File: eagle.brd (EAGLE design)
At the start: 65 x 56 mm, 11 parts, among them IC1 74HCT245, IC2 74HCT245

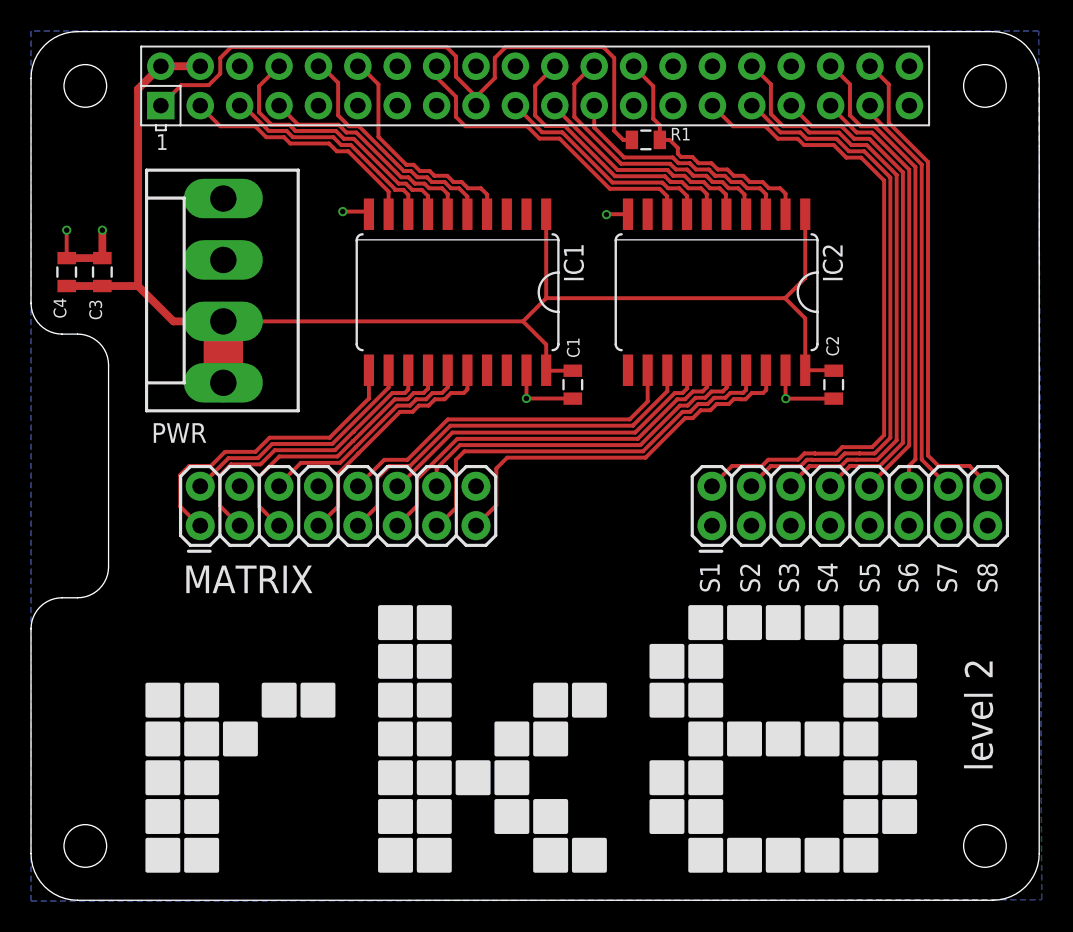
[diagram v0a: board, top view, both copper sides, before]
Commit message: level 3 design
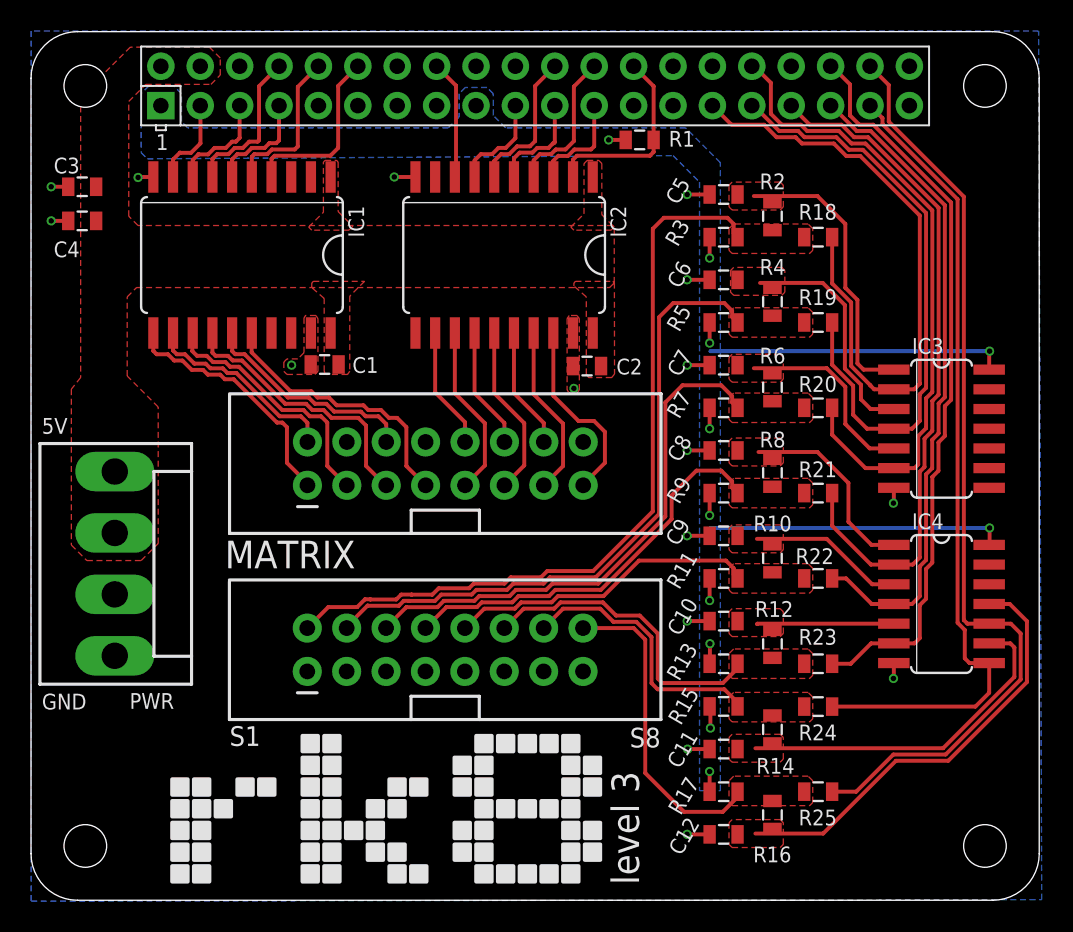
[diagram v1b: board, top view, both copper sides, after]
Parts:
- added C10, C11, C12, C5, C6, C7, C8, C9: 0.1uF, passive:0805
- added IC3, IC4: 74HC14D, 74xx-eu:SO14
- added R10, R11, R12, R13, R14, R15, R16, R17, R2, R3, R4, R5, R6, R7, R8, R9: 10K, passive:0805
- added R18, R19, R20, R21, R22, R23, R24, R25: 0, passive:0805
- J1, J2: device SparkFun-Connectors:2X8 -> SparkFun-Connectors:2X8-SHROUDED_LOCK
- U$1: value RPI3_HATNO_CF -> RPI3_HATNO_DF; device rpi:RASPI_BOARD_B+HAT_DF -> rpi:RASPI_BOARD_B+HAT
- moved J2 19.0 mm to (26.7, 16.1), turned to 90 degrees
- moved PWR 18.9 mm to (5.40, 21.7), turned to 270 degrees
- moved J1 16.3 mm to (26.7, 28.1), turned to 90 degrees
- moved C1 16.1 mm to (18.9, 34.5), turned to 180 degrees
- moved C2 15.9 mm to (35.9, 34.4), turned to 180 degrees
- moved IC1 14.1 mm to (13.6, 41.6)
- moved IC2 13.9 mm to (30.5, 41.6)
- moved C3 5.65 mm to (3.30, 46.0), turned to 180 degrees
- moved C4 3.45 mm to (3.30, 43.8), turned to 180 degrees
- moved R1 0.40 mm to (39.2, 49.0)
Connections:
- removed net S1: J2.2, U$1.29
- removed net S2: J2.4, U$1.31
- removed net S3: J2.6, U$1.32
- removed net S4: J2.8, U$1.33
- removed net S5: J2.10, U$1.35
- removed net S6: J2.12, U$1.36
- removed net S7: J2.14, U$1.37
- removed net S8: J2.16, U$1.38
- new net B1_R: J2.2, R18.1, R2.1, R3.2
- new net B1_S: IC3.2, R18.2, U$1.29
- new net B2_R: J2.4, R19.1, R4.1, R5.2
- new net B2_S: IC3.4, R19.2, U$1.31
- new net B3_R: J2.6, R20.1, R6.1, R7.2
- new net B3_S: IC3.6, R20.2, U$1.32
- new net B4_R: J2.8, R21.1, R8.1, R9.2
- new net B4_S: IC4.2, R21.2, U$1.33
- new net B5_R: J2.10, R10.1, R11.2, R22.1
- new net B5_S: IC4.4, R22.2, U$1.35
- new net B6_R: J2.12, R12.1, R13.2, R23.1
- new net B6_S: IC4.6, R23.2, U$1.36
- new net B7_R: J2.14, R14.1, R15.2, R24.1
- new net B7_S: IC4.8, R24.2, U$1.37
- new net B8_R: J2.16, R16.1, R17.2, R25.1
- new net B8_S: IC4.10, R25.2, U$1.38
- new net N$1: C5.1, IC3.1, R2.2
- new net N$2: C6.1, IC3.3, R4.2
- new net N$3: C7.1, IC3.5, R6.2
- new net N$4: C8.1, IC4.1, R8.2
- new net N$5: C9.1, IC4.3, R10.2
- new net N$6: C10.1, IC4.5, R12.2
- new net N$7: C11.1, IC4.9, R14.2
- new net N$8: C12.1, IC4.11, R16.2
- net +3V3: now also IC3.14, IC4.14, R11.1, R13.1, R15.1, R17.1, R3.1, R5.1, R7.1, R9.1
- net GND: now also C10.2, C11.2, C12.2, C5.2, C6.2, C7.2, C8.2, C9.2, IC3.7, IC4.7
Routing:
- net VCC: track 93.1 -> 0.00 mm
- net B8_S: track 0.00 -> 60.4 mm
- net B7_S: track 0.00 -> 52.3 mm
- net B1_R: track 0.00 -> 50.3 mm
- net B6_S: track 0.00 -> 47.8 mm
- net B4_S: track 0.00 -> 44.3 mm
- net B5_S: track 0.00 -> 42.4 mm
- net B2_R: track 0.00 -> 42.1 mm
- net S1: track 42.0 -> 0.00 mm
- net B3_S: track 0.00 -> 41.7 mm
- net B1_S: track 0.00 -> 41.2 mm
- net B2_S: track 0.00 -> 39.1 mm
- net S3: track 38.6 -> 0.00 mm
- net S2: track 37.9 -> 0.00 mm
- net B3_R: track 0.00 -> 34.3 mm
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- added copper zone on layer 16, net +3V3
- added copper zone on layer 1, net B1_R
- added copper zone on layer 1, net B2_R
- added copper zone on layer 1, net B3_R
- added copper zone on layer 1, net B4_R
- added copper zone on layer 1, net B5_R
- added copper zone on layer 1, net B6_R
- added copper zone on layer 1, net B7_R
- added copper zone on layer 1, net B8_R
- added copper zone on layer 1, net GND
- added copper zone on layer 1, net N$1
- added copper zone on layer 1, net N$2
- added copper zone on layer 1, net N$3
- added copper zone on layer 1, net N$4
- added copper zone on layer 1, net N$5
- added copper zone on layer 1, net N$6
- added copper zone on layer 1, net N$7
- added copper zone on layer 1, net N$8
- added copper zone on layer 1, net VCC
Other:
- outline, holes or cut-outs redrawn
- board text added: "level 3"
- board text removed: "S2"
- board text removed: "S3"
- board text removed: "S4"
- board text removed: "S5"
- board text removed: "S6"
- board text removed: "S7"
- board text removed: "level 2"
